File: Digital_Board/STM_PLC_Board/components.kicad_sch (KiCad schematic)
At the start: 42 parts, among them J2 Conn_02x14_Odd_Even, Q1 2N7002, Q2 2N7002, Q3 2N7002, Q4 2N7002, SW1 SW_Push, SW2 SW_DIP_x01, SW3 SW_DIP_x01

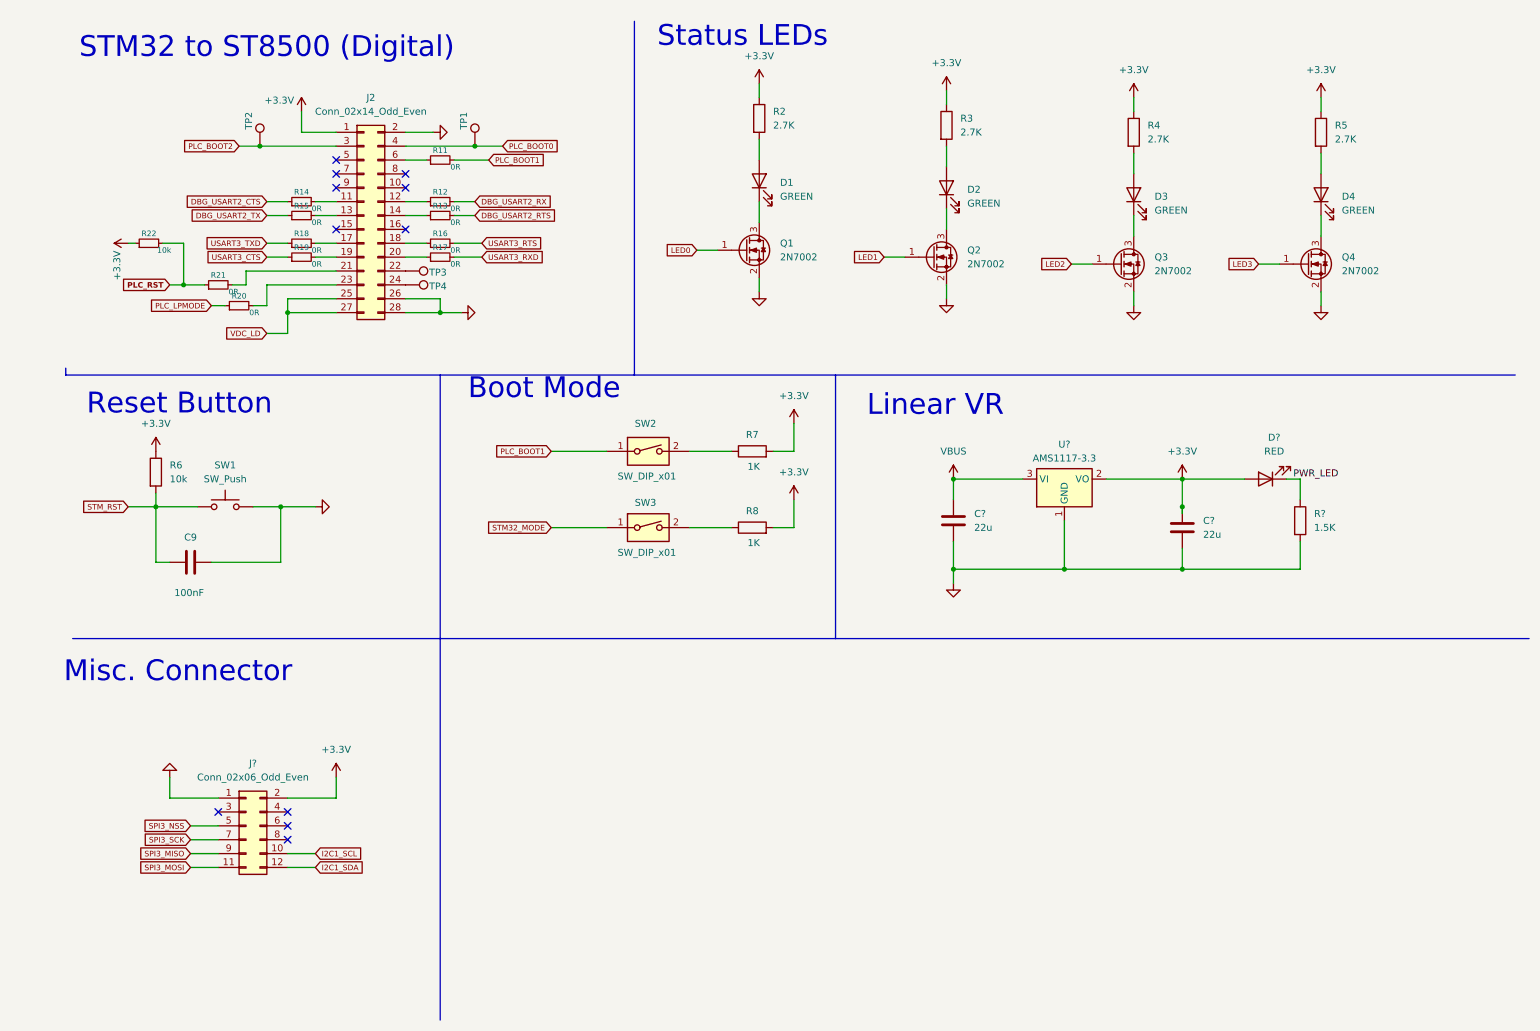
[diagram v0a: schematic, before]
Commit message: schematic done
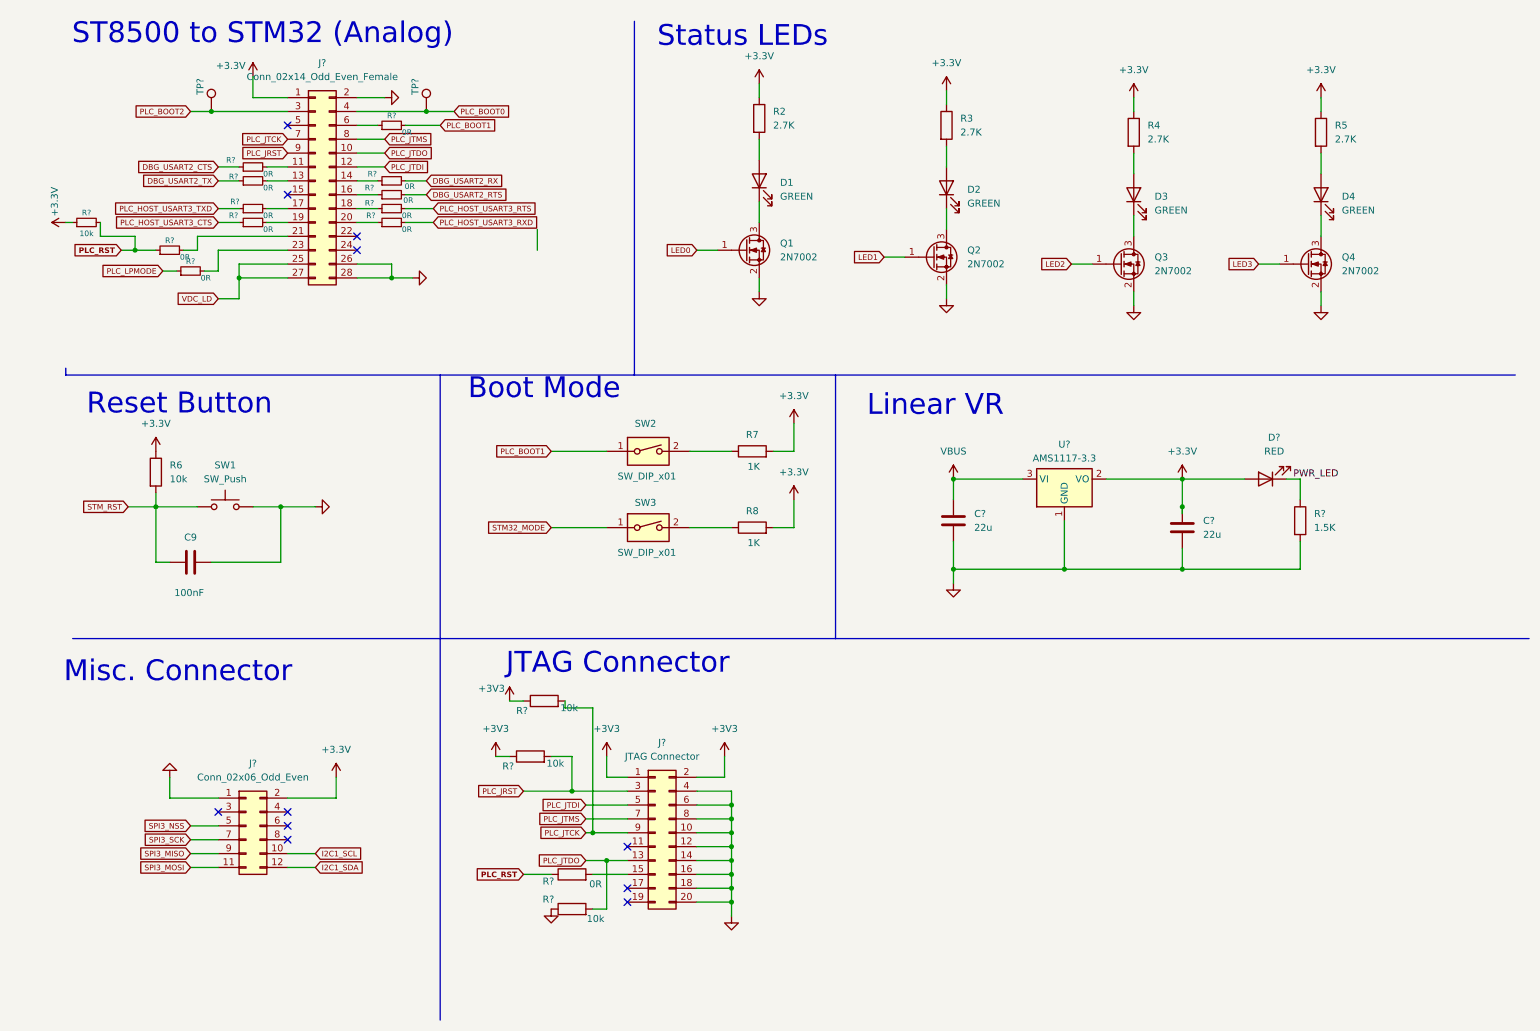
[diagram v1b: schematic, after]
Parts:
- removed J2: Conn_02x14_Odd_Even, symbol Connector_Generic:Conn_02x14_Odd_Even
- removed R11, R12, R13, R14, R15, R16, R17, R18, R19, R20, R21: 0R, symbol Device:R_Small
- removed R22: 10k, symbol Device:R_Small
- removed TP1, TP2, TP3, TP4: TestPoint, symbol Connector:TestPoint
- added J?: Conn_02x14_Odd_Even_Female, symbol Connector_Generic:Conn_02x14_Odd_Even
- added J?: JTAG Connector, symbol Connector_Generic:Conn_02x10_Odd_Even
- added R? (x3): 10k, symbol Device:R
- added R? (x11): 0R, symbol Device:R_Small
- added R?: 0R, symbol Device:R
- added R?: 10k, symbol Device:R_Small
- added TP? (x2): TestPoint, symbol Connector:TestPoint
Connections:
- net +3.3V: now also J?.1 (Pin_1), R?.1
- net DBG_USART2_CTS: now also R?.1
- net DBG_USART2_RTS: now also R?.2
- net DBG_USART2_RX: now also R?.2
- net DBG_USART2_TX: now also R?.1
- net GND: now also J?.10 (Pin_10), J?.12 (Pin_12), J?.14 (Pin_14), J?.16 (Pin_16), J?.18 (Pin_18), J?.2 (Pin_2), J?.20 (Pin_20), J?.26 (Pin_26), J?.28 (Pin_28), J?.4 (Pin_4), J?.6 (Pin_6), J?.8 (Pin_8), R?.1
- net PLC_BOOT0: now also J?.4 (Pin_4), TP?.1
- net PLC_BOOT1: now also R?.2
- net PLC_BOOT2: now also J?.3 (Pin_3), TP?.1
- net PLC_LPMODE: now also R?.1
- net PLC_RST: now also R?.1, R?.1, R?.2
- net VDC_LD: now also J?.25 (Pin_25), J?.27 (Pin_27)
- new net: J?.21 (Pin_21), R?.2
- new net: J?.11 (Pin_11), R?.2
- new net: J?.13 (Pin_13), R?.2
- new net: J?.14 (Pin_14), R?.1
- new net: J?.16 (Pin_16), R?.1
- new net: J?.17 (Pin_17), R?.2
- new net: J?.18 (Pin_18), R?.1
- new net: J?.19 (Pin_19), R?.2
- new net: J?.20 (Pin_20), R?.1
- new net: J?.23 (Pin_23), R?.2
- new net: J?.6 (Pin_6), R?.1
- new net: J?.15 (Pin_15), R?.2
- new net +3V3: J?.1 (Pin_1), J?.2 (Pin_2), R?.1, R?.1
- new net PLC_HOST_USART3_CTS: R?.1
- new net PLC_HOST_USART3_RTS: R?.2
- new net PLC_HOST_USART3_RXD: R?.2
- new net PLC_HOST_USART3_TXD: R?.1
- new net PLC_JRST: J?.3 (Pin_3), J?.9 (Pin_9), R?.2
- new net PLC_JTCK: J?.7 (Pin_7), J?.9 (Pin_9), R?.2
- new net PLC_JTDI: J?.12 (Pin_12), J?.5 (Pin_5)
- new net PLC_JTDO: J?.10 (Pin_10), J?.13 (Pin_13), R?.2
- new net PLC_JTMS: J?.7 (Pin_7), J?.8 (Pin_8)
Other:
- note added: "JTAG Connector"
- note added: "ST8500 to STM32 (Analog)"
- note removed: "STM32 to ST8500 (Digital)"
